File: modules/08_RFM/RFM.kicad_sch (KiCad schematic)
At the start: 53 parts, among them IC1 LF356_Swap, IC2 TL074, IC3 TL074, P1 47k, P10 47k, P2 47k, P3 10k, P4 47k, P5 47k, P6 10k

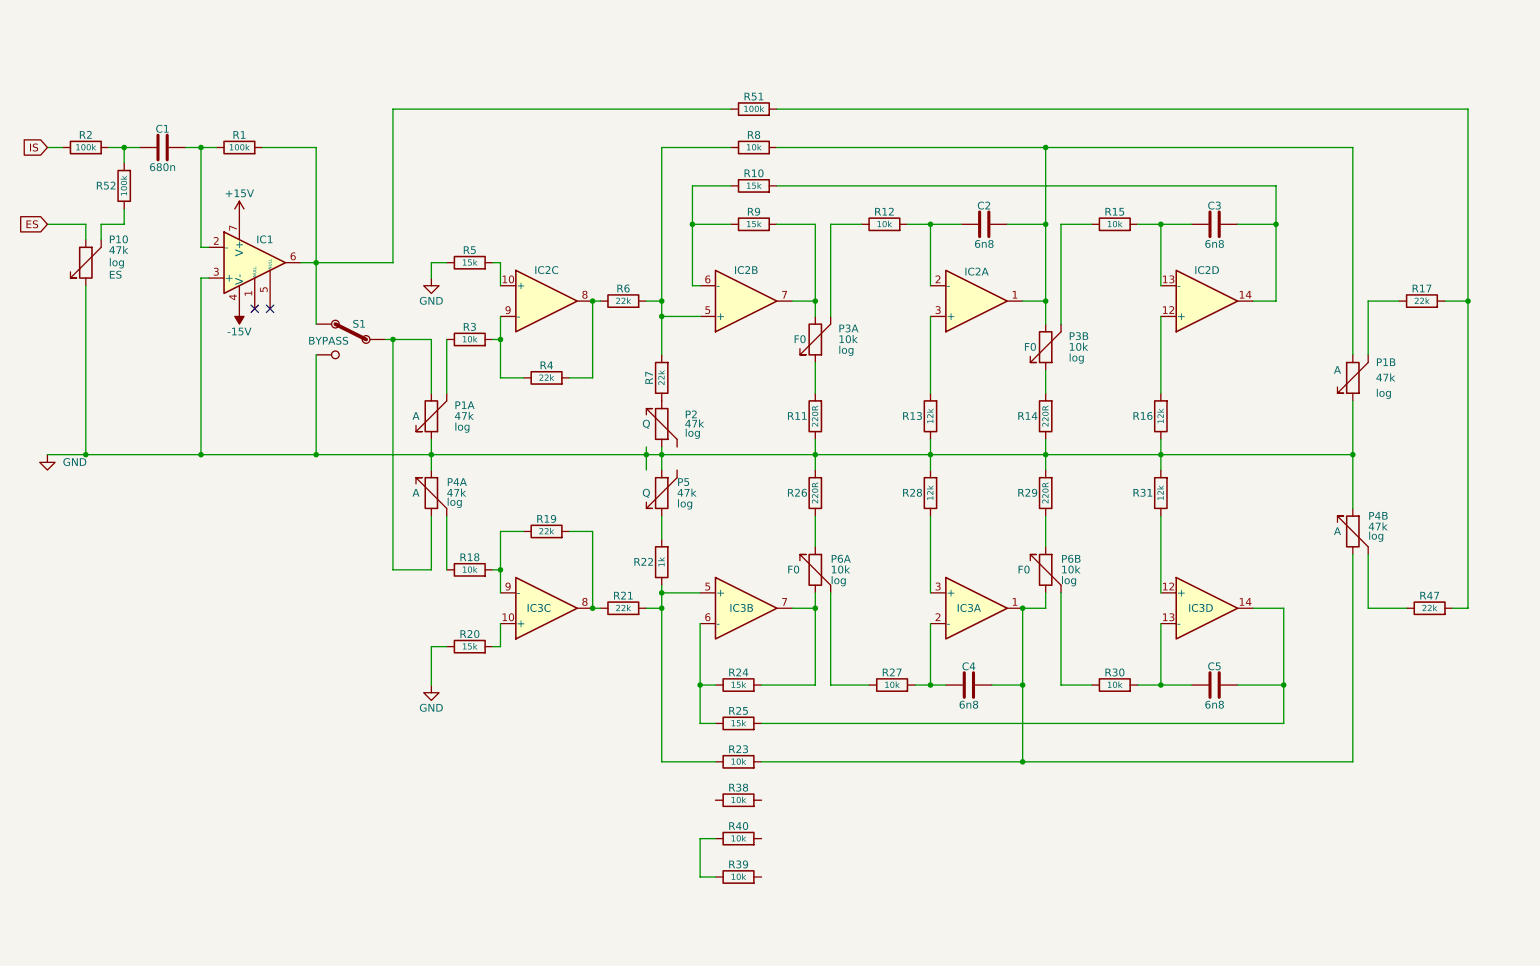
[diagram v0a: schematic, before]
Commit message: rfm work
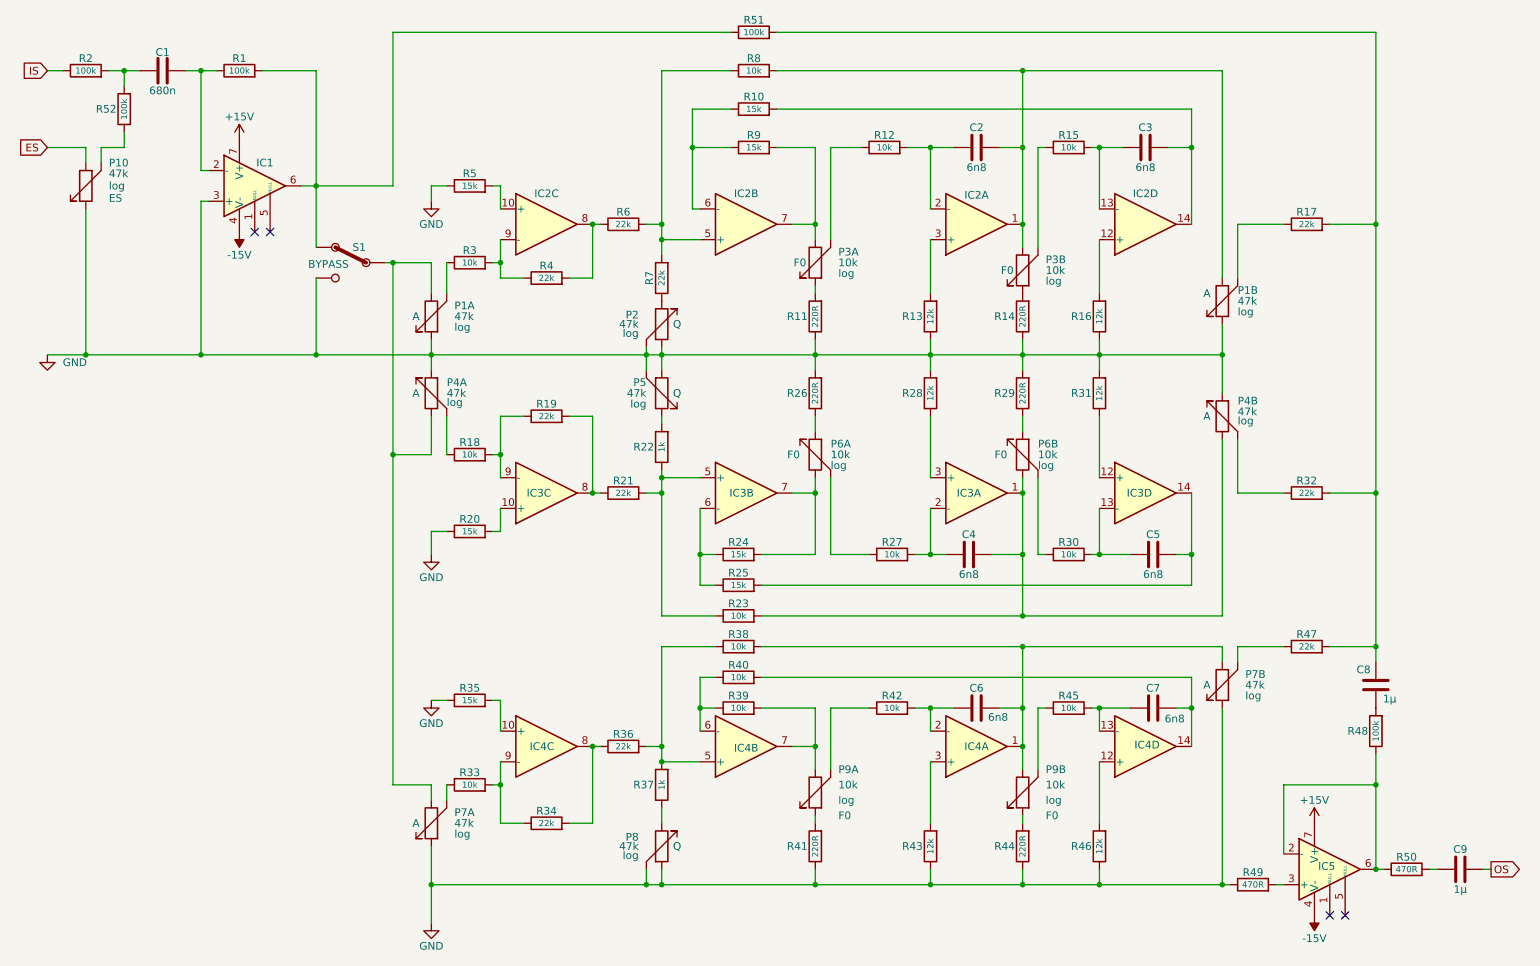
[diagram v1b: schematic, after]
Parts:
- added C6, C7: 6n8, FormantKO:C_Disc_300_400, symbol FormantKO:C
- added C8, C9: 1µ, FormantKO:C_Disc_300_400, symbol FormantKO:C
- added IC4: TL074, FormantKO:DIP-14, symbol FormantKO:TL074
- added IC5: LF357_Swap, FormantKO:DIP-8, symbol FormantKO:LF357_Swap
- added P7: 47k, FormantKO:Panel_Connector_1x06, symbol FormantKO:R_Potentiometer_Dual
- added P8: 47k, FormantKO:Panel_Connector_1x03, symbol FormantKO:R_Potentiometer
- added P9: 10k, FormantKO:Panel_Connector_1x06, symbol FormantKO:R_Potentiometer_Dual
- added R33, R42, R45: 10k, FormantKO:R_Axial_Horizontal, symbol FormantKO:R
- added R34, R36, R47: 22k, FormantKO:R_Axial_Horizontal, symbol FormantKO:R
- added R35: 15k, FormantKO:R_Axial_Horizontal, symbol FormantKO:R
- added R37: 1k, FormantKO:R_Axial_Horizontal, symbol FormantKO:R
- added R41, R44: 220R, FormantKO:R_Axial_Horizontal, symbol FormantKO:R
- added R43, R46: 12k, FormantKO:R_Axial_Horizontal, symbol FormantKO:R
- added R48: 100k, FormantKO:R_Axial_Horizontal, symbol FormantKO:R
- added R49, R50: 470R, FormantKO:R_Axial_Horizontal, symbol FormantKO:R
- C1, C2, C3, C4, C5: footprint FormantKO:C_Disc -> FormantKO:C_Disc_300_400
- P1, P3, P4, P6: symbol FormantKO:Panel_Dual_Potentiometer_6 -> FormantKO:R_Potentiometer_Dual
- P10, P2, P5: symbol FormantKO:Panel_Potentiometer_3 -> FormantKO:R_Potentiometer
- S1: symbol FormantKO:SWITCH_SPDT -> FormantKO:SW_SPDT
- renumbered R47 to R32
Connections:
- net +15V: now also IC5.7 (V+)
- net -15V: now also IC5.4 (V-)
- net GND: now also P2.2, P5.2, P7.1, P7.4, P8.2, P8.3, R35.1, R41.1, R43.1, R44.1, R46.1, R49.1
- net at P1.3, P4.3, S1.2 (c): now also P7.3
- net at R17.2, R32.2, R51.2: now also C8.2, R47.2
- net at IC2.1, P1.6, P3.6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: now also C2.1; no longer C2.2
- net at IC3.2 (-), R27.2: now also C4.2; no longer C4.1
- net at R38.1: now also IC4.5 (+), R36.2, R37.2
- net at R38.2: now also C6.1, IC4.1, P7.6, P9.6
- net at IC2.13 (-), R15.2: now also C3.2; no longer C3.1
- net at IC2.14, R10.2: now also C3.1; no longer C3.2
- net at IC3.1, P4.6, P6.6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: now also C4.1; no longer C4.2
- net at IC3.14, R25.2: now also C5.1; no longer C5.2
- net at R39.1, R40.1: now also IC4.6 (-)
- net at R39.2: now also IC4.7, P9.3
- net at IC2.2 (-), R12.2: now also C2.2; no longer C2.1
- net at IC3.13 (-), R30.2: now also C5.2; no longer C5.1
- net at R40.2: now also C7.1, IC4.14
- new net: IC4.10 (+), R35.2
- new net: IC4.12 (+), R46.2
- new net: C7.2, IC4.13 (-), R45.2
- new net: P7.5, R47.1
- new net: IC5.3 (+), R49.2
- new net: IC5.2 (-), IC5.6, R48.1, R50.1
- new net: C9.2, R50.2
- new net: P9.1, R41.2
- new net: P9.2, R42.1
- new net: P9.5, R45.1
- new net: C6.2, IC4.2 (-), R42.2
- new net: C8.1, R48.2
- new net: IC4.3 (+), R43.2
- new net: P8.1, R37.1
- new net: IC4.8, R34.2, R36.1
- new net: IC4.9 (-), R33.2, R34.1
- new net: P9.4, R44.2
- new net: P7.2, R33.1
- new net OS: C9.1
- no-connect marks 2 -> 4
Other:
- moved on the sheet: C1, C2, C3, C4, C5, IC1, IC2A, IC2B, IC2C, IC2D, IC3A, IC3B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

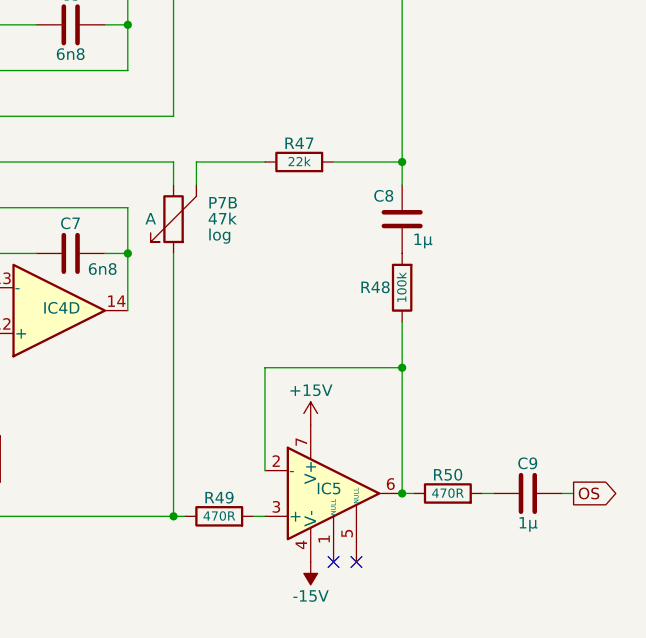
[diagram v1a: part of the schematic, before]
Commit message: rfm tracks
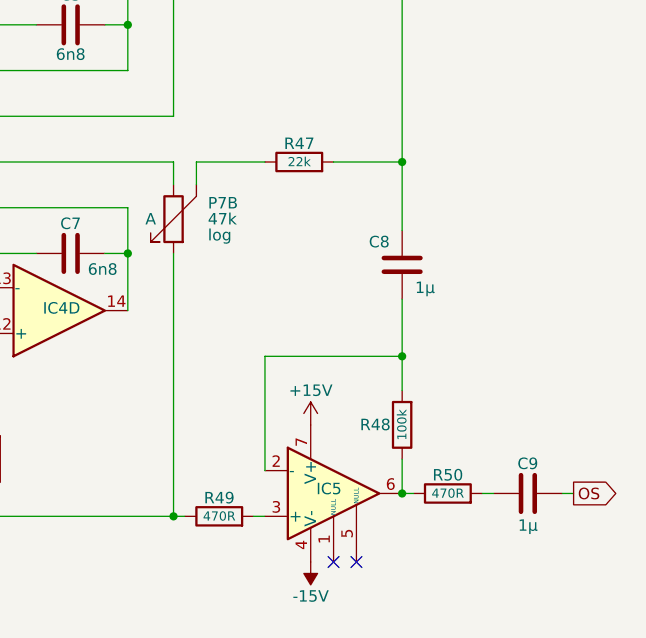
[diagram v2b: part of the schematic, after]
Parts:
- C8, C9: footprint FormantKO:C_Disc_300_400 -> FormantKO:C_Rect_400_600
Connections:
- net OS: now also C9.2; no longer C9.1
- net at R17.2, R32.2, R47.2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: now also C8.1; no longer C8.2
- net at IC5.6, R48.1, R50.1: no longer IC5.2 (-)
- net at R50.2: now also C9.1; no longer C9.2
- net at R48.2: now also C8.2, IC5.2 (-); no longer C8.1
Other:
- moved on the sheet: C8, C9, R48
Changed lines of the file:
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@@
 	)
 	(junction
-		(at 238.76 143.51)
+		(at 193.04 105.41)
 		(diameter 0)
 		(color 0 0 0 0)
 	)
 	(junction
-		(at 193.04 105.41)
+		(at 146.05 50.8)
 		(diameter 0)
 		(color 0 0 0 0)
 	)
 	(junction
-		(at 146.05 50.8)
+		(at 165.1 72.39)
 		(diameter 0)
 		(color 0 0 0 0)
 	)
 	(junction
-		(at 165.1 72.39)
+		(at 238.76 157.48)
 		(diameter 0)
 		(color 0 0 0 0)
@@
 	)
 	(junction
-		(at 238.76 120.65)
-		(diameter 0)
-		(color 0 0 0 0)
-	)
-	(junction
 		(at 208.28 130.81)
 		(diameter 0)
@@
 	)
 	(junction
-		(at 238.76 157.48)
+		(at 125.73 38.1)
 		(diameter 0)
 		(color 0 0 0 0)
 	)
 	(junction
-		(at 125.73 38.1)
+		(at 31.75 25.4)
 		(diameter 0)
 		(color 0 0 0 0)
 	)
 	(junction
-		(at 31.75 25.4)
+		(at 238.76 120.65)
 		(diameter 0)
 		(color 0 0 0 0)
@@
 	)
 	(junction
+		(at 238.76 142.24)
+		(diameter 0)
+		(color 0 0 0 0)
+	)
+	(junction
 		(at 165.1 160.02)
 		(diameter 0)
@@
 	(wire
 		(pts
-			(xy 223.52 154.94) (xy 223.52 143.51)
+			(xy 223.52 154.94) (xy 223.52 142.24)
 		)
 		(stroke
@@
 	(wire
 		(pts
+			(xy 238.76 135.89) (xy 238.76 142.24)
+		)
+		(stroke
+			(width 0)
+			(type default)
+		)
+	)
+	(wire
+		(pts
 			(xy 180.34 105.41) (xy 175.26 105.41)
 		)
@@
 	(wire
 		(pts
-			(xy 223.52 143.51) (xy 238.76 143.51)
+			(xy 223.52 142.24) (xy 238.76 142.24)
 		)
 		(stroke
@@
 	(wire
 		(pts
-			(xy 238.76 143.51) (xy 238.76 157.48)
-		)
-		(stroke
-			(width 0)
-			(type default)
-		)
-	)
-	(wire
-		(pts
 			(xy 120.65 120.65) (xy 120.65 137.16)
 		)
@@
 	(wire
 		(pts
+			(xy 238.76 153.67) (xy 238.76 157.48)
+		)
+		(stroke
+			(width 0)
+			(type default)
+		)
+	)
+	(wire
+		(pts
 			(xy 120.65 91.44) (xy 120.65 92.71)
 		)
@@
 	(wire
 		(pts
-			(xy 238.76 138.43) (xy 238.76 143.51)
-		)
-		(stroke
-			(width 0)
-			(type default)
-		)
-	)
-	(wire
-		(pts
 			(xy 193.04 130.81) (xy 193.04 134.62)
 		)
@@
 	(wire
 		(pts
+			(xy 238.76 142.24) (xy 238.76 146.05)
+		)
+		(stroke
+			(width 0)
+			(type default)
+		)
+	)
+	(wire
+		(pts
 			(xy 193.04 72.39) (xy 193.04 74.93)
 		)
@@
 	(wire
 		(pts
-			(xy 238.76 120.65) (xy 238.76 123.19)
+			(xy 238.76 120.65) (xy 238.76 128.27)
 		)
 		(stroke
@@
 	(symbol
 		(lib_id "FormantKO:C")
-		(at 252.73 157.48 270)
+		(at 252.73 157.48 90)
 		(unit 1)
 		(body_style 1)
@@
 		)
 		(property "Value" "1µ"
-			(at 252.73 160.782 90)
+			(at 252.73 161.036 90)
 			(show_name no)
 			(do_not_autoplace no)
@@
 			)
 		)
-		(property "Footprint" "FormantKO:C_Disc_300_400"
+		(property "Footprint" "FormantKO:C_Rect_400_600"
 			(at 252.73 157.48 0)
 			(hide yes)
@@
 	(symbol
 		(lib_id "FormantKO:R")
-		(at 238.76 134.62 90)
+		(at 238.76 149.86 90)
 		(unit 1)
 		(body_style 1)
@@
 		(dnp no)
 		(property "Reference" "R48"
-			(at 237.49 134.62 90)
+			(at 237.49 149.86 90)
 			(show_name no)
 			(do_not_autoplace no)
@@
 		)
 		(property "Value" "100k"
-			(at 238.76 134.62 0)
+			(at 238.76 149.86 0)
 			(show_name no)
 			(do_not_autoplace no)
@@
 		)
 		(property "Footprint" "FormantKO:R_Axial_Horizontal"
-			(at 238.76 134.62 0)
+			(at 238.76 149.86 0)
 			(hide yes)
 			(show_name no)
@@
 		)
 		(property "Datasheet" ""
-			(at 238.76 134.62 90)
+			(at 238.76 149.86 90)
 			(hide yes)
 			(show_name no)
@@
 		)
 		(property "Description" "Resistor"
-			(at 238.76 134.62 0)
+			(at 238.76 149.86 0)
 			(hide yes)
 			(show_name no)
@@
 	(symbol
 		(lib_id "FormantKO:C")
-		(at 238.76 127 180)
+		(at 238.76 132.08 0)
 		(unit 1)
 		(body_style 1)
@@
 		(dnp no)
 		(property "Reference" "C8"
-			(at 236.728 124.46 0)
+			(at 236.22 129.54 0)
 			(show_name no)
 			(do_not_autoplace no)
@@
 		)
 		(property "Value" "1µ"
-			(at 241.046 129.286 0)
+			(at 241.3 134.62 0)
 			(show_name no)
 			(do_not_autoplace no)
@@
 			)
 		)
-		(property "Footprint" "FormantKO:C_Disc_300_400"
-			(at 238.76 127 0)
+		(property "Footprint" "FormantKO:C_Rect_400_600"
+			(at 238.76 132.08 0)
 			(hide yes)
 			(show_name no)
@@
 		)
 		(property "Datasheet" ""
-			(at 238.76 127 0)
+			(at 238.76 132.08 0)
 			(hide yes)
 			(show_name no)
@@
 		)
 		(property "Description" "Unpolarized capacitor"
-			(at 238.76 127 0)
+			(at 238.76 132.08 0)
 			(hide yes)
 			(show_name no)

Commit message: rfm routing
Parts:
- IC1: value LF356_Swap -> LF356
- IC5: value LF357_Swap -> LF357
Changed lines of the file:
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@@
 			)
 		)
-		(property "Value" "LF357_Swap"
+		(property "Value" "LF357"
 			(at 243.84 153.5998 0)
 			(hide yes)
@@
 			)
 		)
-		(property "Value" "LF356_Swap"
+		(property "Value" "LF356"
 			(at 53.34 40.64 0)
 			(hide yes)
